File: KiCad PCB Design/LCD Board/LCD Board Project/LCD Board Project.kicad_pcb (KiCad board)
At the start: 2 copper layers, 22.2 x 14 mm, 8 parts, among them J1 Conn_01x03_Male, J2 Conn_01x03_Male, J3 Conn_01x02_Male, U1 ATtiny412-SS

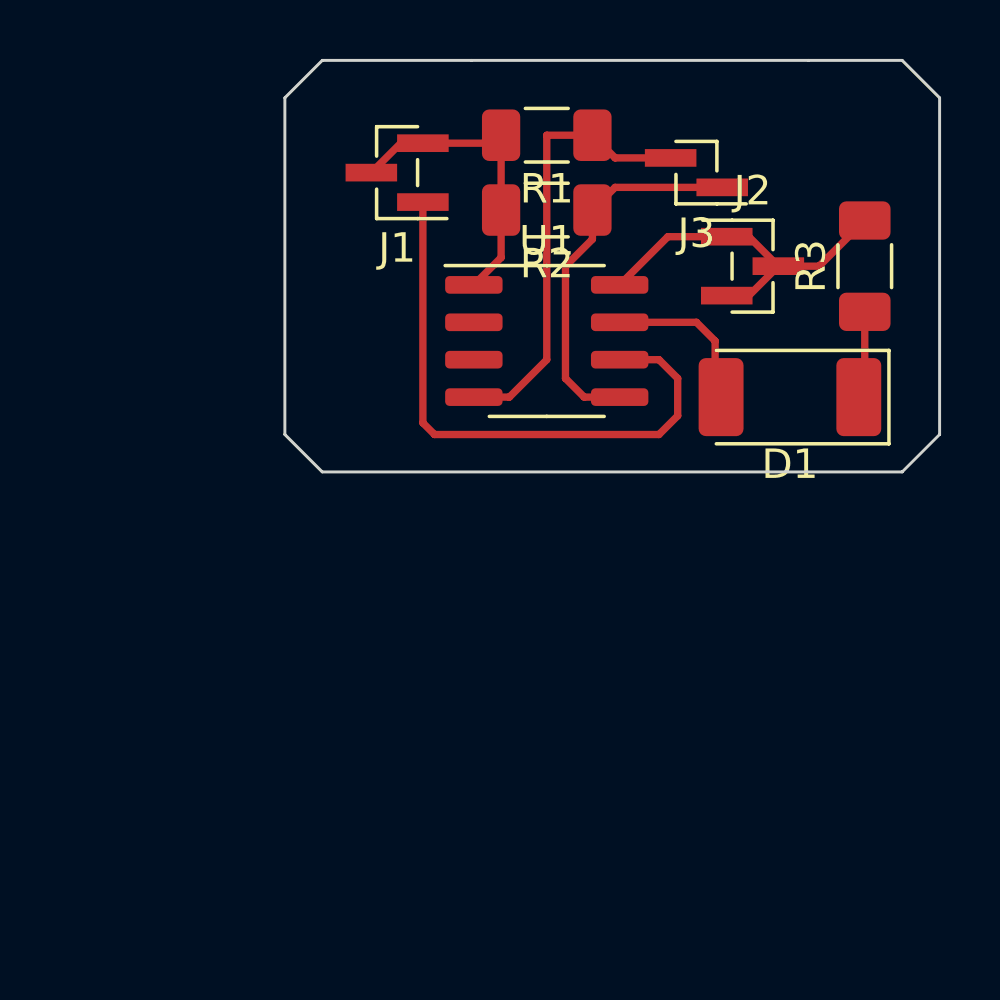
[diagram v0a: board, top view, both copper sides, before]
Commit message: v1.4 - Unknown Updates
Not sure what was changed but I want to push updates.
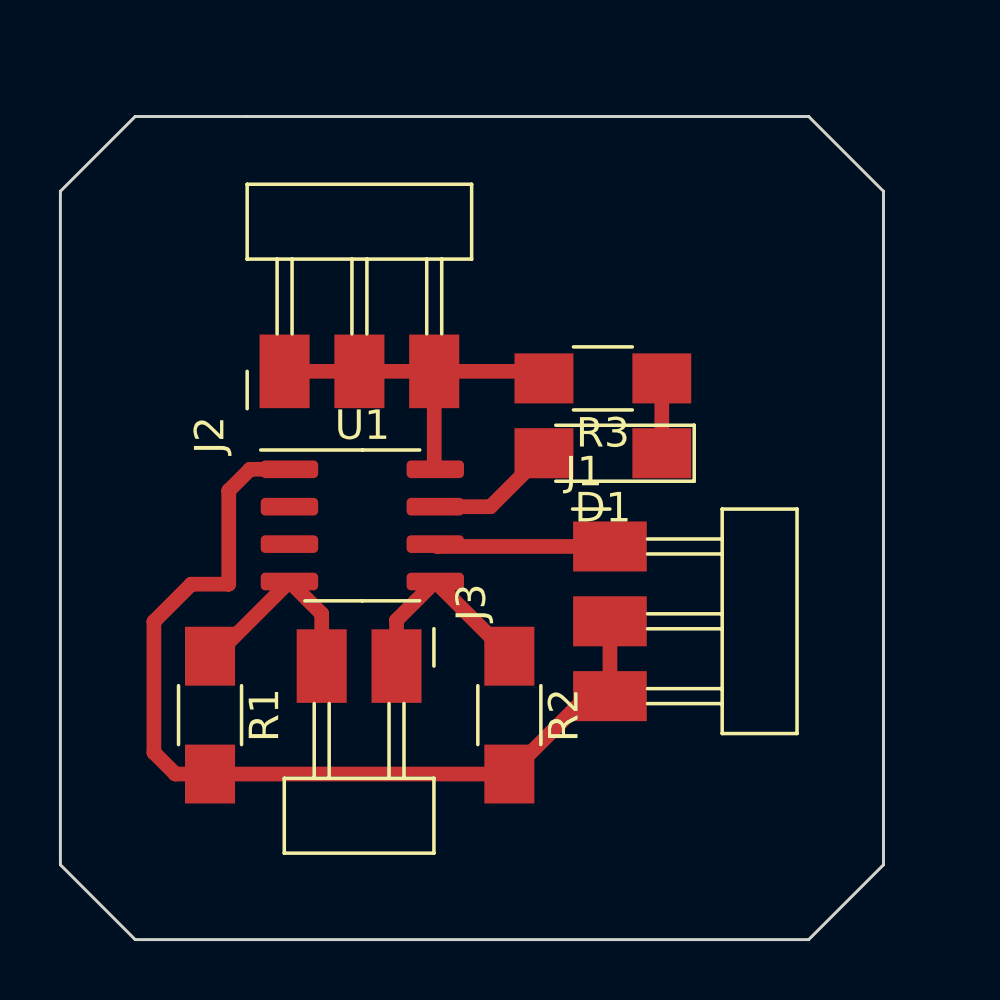
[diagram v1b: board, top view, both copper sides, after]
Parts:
- D1: footprint LED_SMD:LED_2010_5025Metric_Pad1.52x2.65mm_HandSolder -> fab:LED_1206
- J1, J2: footprint Connector_PinHeader_1.00mm:PinHeader_1x03_P1.00mm_Vertical_SMD_Pin1Left -> fab:PinHeader_1x03_P2.54mm_Horizontal_SMD
- J3: footprint Connector_PinHeader_1.00mm:PinHeader_1x02_P1.00mm_Vertical_SMD_Pin1Left -> fab:PinHeader_1x02_P2.54mm_Horizontal_SMD
- R1, R2, R3: footprint Resistor_SMD:R_1206_3216Metric_Pad1.30x1.75mm_HandSolder -> fab:R_1206
- moved R1 22.8 mm to (135.9, 114.3), turned to -90 degrees
- moved J3 19.6 mm to (142.2, 112.6), turned to -90 degrees
- moved R2 17.2 mm to (146.1, 114.3), turned to -90 degrees
- moved J2 16.3 mm to (138.4, 102.6), turned to 90 degrees
- moved J1 14.6 mm to (149.5, 108.6), turned to 0 degrees
- moved R3 9.67 mm to (149.2, 102.9), turned to 180 degrees
- moved U1 8.85 mm to (141.1, 107.9)
- moved D1 6.63 mm to (149.2, 105.4)
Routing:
- net Net-(J1-Pad2): track 10.4 -> 32.5 mm
- net Net-(J1-Pad1): track 20.1 -> 5.96 mm
- net Net-(J3-Pad2): track 15.1 -> 7.07 mm
- net Net-(J3-Pad1): track 12.9 -> 6.99 mm
- net Net-(D1-Pad2): track 5.49 -> 4.44 mm
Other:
- board size 22.2 x 14 mm -> 27.9 x 27.9 mm
